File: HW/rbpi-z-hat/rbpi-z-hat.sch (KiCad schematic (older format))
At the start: 4 parts

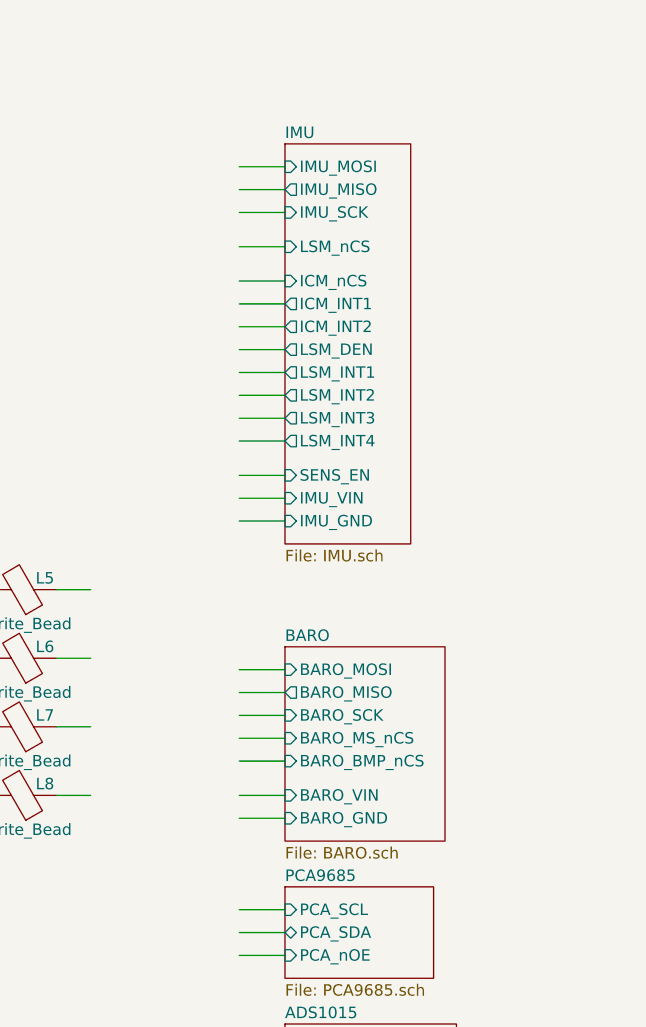
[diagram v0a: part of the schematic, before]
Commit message: Commit
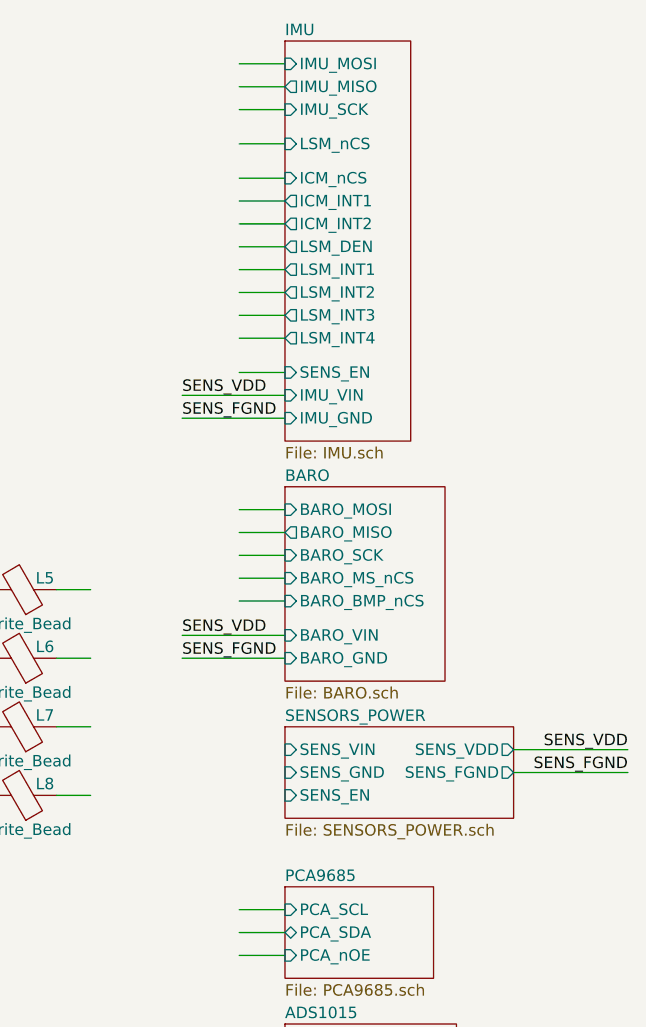
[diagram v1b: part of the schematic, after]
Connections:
- net labels added: SENS_FGND, SENS_VDD
- wire segments 67 -> 69
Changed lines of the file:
@@
 	4350 4050 4200 4050
 $Sheet
-S 5200 3400 700  850
+S 5200 2700 700  850
 U 5EF65A4D
 F0 "BARO" 50
 F1 "BARO.sch" 50
-F2 "BARO_VIN" I L 5200 4050 50
-F3 "BARO_MOSI" I L 5200 3500 50
-F4 "BARO_MISO" O L 5200 3600 50
-F5 "BARO_SCK" I L 5200 3700 50
-F6 "BARO_MS_nCS" I L 5200 3800 50
-F7 "BARO_BMP_nCS" I L 5200 3900 50
-F8 "BARO_GND" I L 5200 4150 50
+F2 "BARO_VIN" I L 5200 3350 50
+F3 "BARO_MOSI" I L 5200 2800 50
+F4 "BARO_MISO" O L 5200 2900 50
+F5 "BARO_SCK" I L 5200 3000 50
+F6 "BARO_MS_nCS" I L 5200 3100 50
+F7 "BARO_BMP_nCS" I L 5200 3200 50
+F8 "BARO_GND" I L 5200 3450 50
 $EndSheet
 $Sheet
@@
 	4700 8000 5200 8000
 $Sheet
-S 5200 1200 550  1750
+S 5200 750  550  1750
 U 5EE06F22
 F0 "IMU" 50
 F1 "IMU.sch" 50
-F2 "IMU_VIN" I L 5200 2750 50
-F3 "IMU_GND" I L 5200 2850 50
-F4 "IMU_MOSI" I L 5200 1300 50
-F5 "IMU_MISO" O L 5200 1400 50
-F6 "IMU_SCK" I L 5200 1500 50
-F7 "LSM_nCS" I L 5200 1650 50
-F8 "ICM_nCS" I L 5200 1800 50
-F9 "ICM_INT1" O L 5200 1900 50
-F10 "ICM_INT2" O L 5200 2000 50
-F11 "LSM_DEN" O L 5200 2100 50
-F12 "LSM_INT1" O L 5200 2200 50
-F13 "LSM_INT2" O L 5200 2300 50
-F14 "LSM_INT3" O L 5200 2400 50
-F15 "LSM_INT4" O L 5200 2500 50
-F16 "SENS_EN" I L 5200 2650 50
-$EndSheet
-Wire Wire Line
-	5200 1300 5000 1300
-Wire Wire Line
-	5200 1400 5000 1400
-Wire Wire Line
-	5200 1500 5000 1500
+F2 "IMU_VIN" I L 5200 2300 50
+F3 "IMU_GND" I L 5200 2400 50
+F4 "IMU_MOSI" I L 5200 850 50
+F5 "IMU_MISO" O L 5200 950 50
+F6 "IMU_SCK" I L 5200 1050 50
+F7 "LSM_nCS" I L 5200 1200 50
+F8 "ICM_nCS" I L 5200 1350 50
+F9 "ICM_INT1" O L 5200 1450 50
+F10 "ICM_INT2" O L 5200 1550 50
+F11 "LSM_DEN" O L 5200 1650 50
+F12 "LSM_INT1" O L 5200 1750 50
+F13 "LSM_INT2" O L 5200 1850 50
+F14 "LSM_INT3" O L 5200 1950 50
+F15 "LSM_INT4" O L 5200 2050 50
+F16 "SENS_EN" I L 5200 2200 50
+$EndSheet
+Wire Wire Line
+	5200 850  5000 850
+Wire Wire Line
+	5200 950  5000 950
+Wire Wire Line
+	5200 1050 5000 1050
+Wire Wire Line
+	5200 1200 5000 1200
+Wire Wire Line
+	5200 1350 5000 1350
+Wire Wire Line
+	5200 1450 5000 1450
+Wire Wire Line
+	5200 1550 5000 1550
 Wire Wire Line
 	5200 1650 5000 1650
 Wire Wire Line
-	5200 1800 5000 1800
-Wire Wire Line
-	5200 1900 5000 1900
-Wire Wire Line
-	5200 2000 5000 2000
-Wire Wire Line
-	5200 2100 5000 2100
+	5200 1750 5000 1750
+Wire Wire Line
+	5200 1850 5000 1850
+Wire Wire Line
+	5200 1950 5000 1950
+Wire Wire Line
+	5200 2050 5000 2050
 Wire Wire Line
 	5200 2200 5000 2200
 Wire Wire Line
-	5200 2300 5000 2300
-Wire Wire Line
-	5200 2400 5000 2400
-Wire Wire Line
-	5200 2500 5000 2500
-Wire Wire Line
-	5200 2650 5000 2650
-Wire Wire Line
-	5200 2750 5000 2750
-Wire Wire Line
-	5200 2850 5000 2850
-Wire Wire Line
-	5200 3500 5000 3500
-Wire Wire Line
-	5200 3600 5000 3600
-Wire Wire Line
-	5200 3700 5000 3700
-Wire Wire Line
-	5200 3800 5000 3800
-Wire Wire Line
-	5200 3900 5000 3900
-Wire Wire Line
-	5200 4050 5000 4050
-Wire Wire Line
-	5200 4150 5000 4150
+	5200 2300 4750 2300
+Wire Wire Line
+	5200 2400 4750 2400
+Wire Wire Line
+	5200 2800 5000 2800
+Wire Wire Line
+	5200 2900 5000 2900
+Wire Wire Line
+	5200 3000 5000 3000
+Wire Wire Line
+	5200 3100 5000 3100
+Wire Wire Line
+	5200 3200 5000 3200
+Wire Wire Line
+	5200 3350 4750 3350
 Wire Wire Line
 	5200 4550 5000 4550
@@
 Text Label 3350 3000 2    50   ~ 0
 SCL1
+$Sheet
+S 5200 3750 1000 400
+U 5EE7A13E
+F0 "SENSORS_POWER" 50
+F1 "SENSORS_POWER.sch" 50
+F2 "SENS_VIN" I L 5200 3850 50
+F3 "SENS_GND" I L 5200 3950 50
+F4 "SENS_EN" I L 5200 4050 50
+F5 "SENS_VDD" O R 6200 3850 50
+F6 "SENS_FGND" O R 6200 3950 50
+$EndSheet
+Wire Wire Line
+	6200 3850 6700 3850
+Text Label 6700 3850 2    50   ~ 0
+SENS_VDD
+Text Label 4750 2300 0    50   ~ 0
+SENS_VDD
+Text Label 4750 3350 0    50   ~ 0
+SENS_VDD
+Wire Wire Line
+	6200 3950 6700 3950
+Text Label 6700 3950 2    50   ~ 0
+SENS_FGND
+Text Label 4750 2400 0    50   ~ 0
+SENS_FGND
+Wire Wire Line
+	5200 3450 4750 3450
+Text Label 4750 3450 0    50   ~ 0
+SENS_FGND
 $EndSCHEMATC
